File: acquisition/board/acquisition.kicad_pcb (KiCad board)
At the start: 4 copper layers, 432 parts, among them J1 XILINX_JTAG, J10 MMCX, J11 MMCX, J12 MMCX, J13 MMCX, J14 MMCX, J15 MMCX, J16 MMCX, J17 MMCX, J18 UX60SX-MB-5ST, J19 CONN_01X05, J2 MMCX, J20 CONN_01X06, J3 MMCX, J4 MMCX, J5 MMCX, J6 MMCX, J7 MMCX, J8 MMCX, J9 MMCX, Q1 SSM6N58NU, Q2 SSM6N58NU, U1 AD9251, U10 FT232HL, U11 LMK04806, U12 AK5DAF1-100.0000T2, U14 74AVCH1T45, U15 74AVCH1T45, U16 74AVCH1T45, U17 74AVCH1T45, U18 74AVCH1T45, U19 74AVCH1T45, U2 XC7A50T-1FTG256C, U20 74AVCH1T45, U21 ECS-3225MVQ-120-CN-TR, U22 93LC56B-MS, U23 74AVCH1T45, U24 74AVCH1T45, U25 LTC3374-QFN, U26 LT3042, U27 LT3042, U28 ADR510, U29 SIP32408, U3 AD9251, U30 LDO1117-12, U4 AD9251, U5 AD9251, U6 ICE40UP5K_QFN48, U7 STM32L031-QFN32, U8 S27KS0642, U9 S25FL128SAGBHIA10

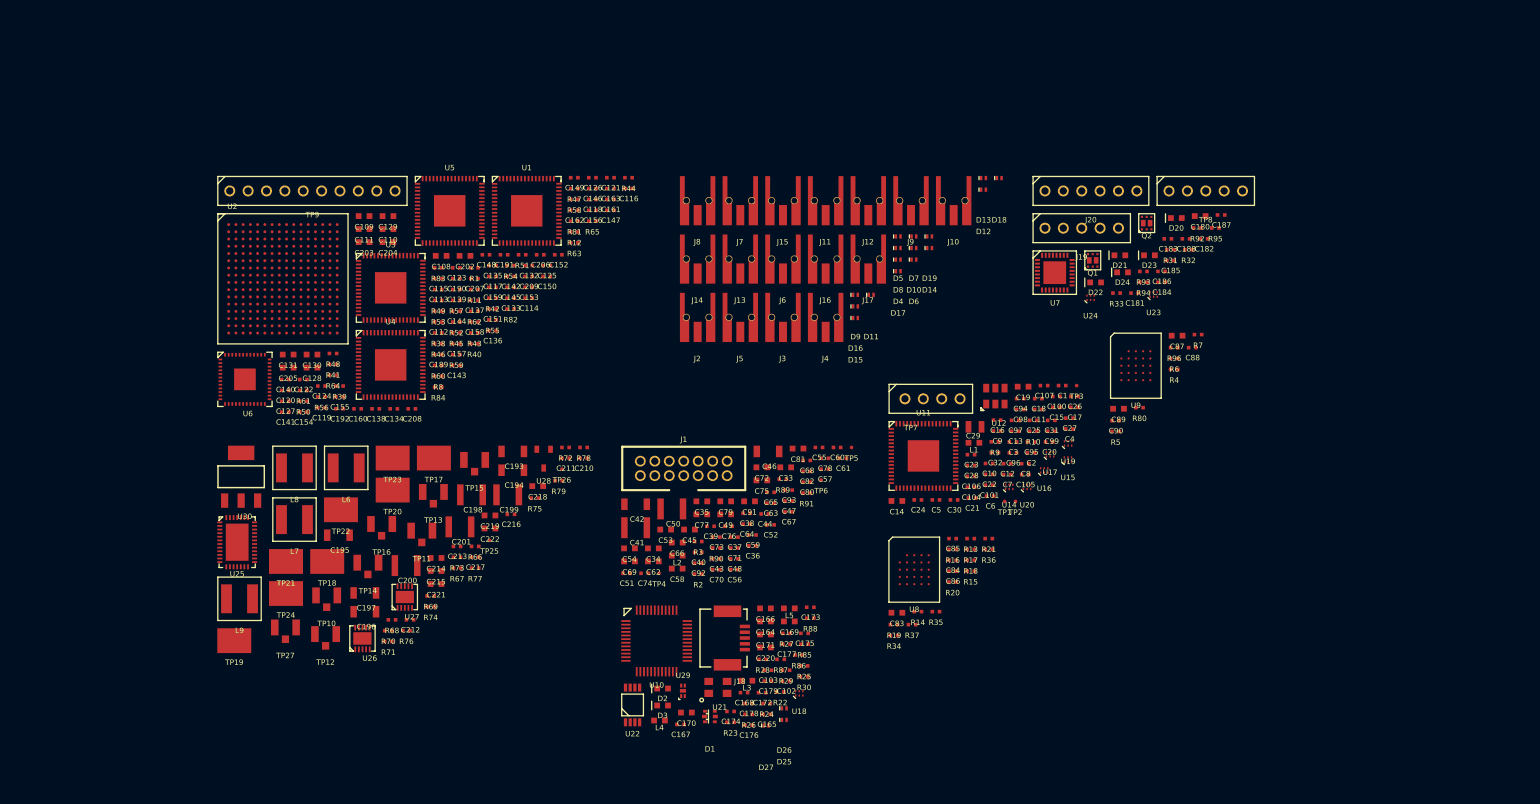
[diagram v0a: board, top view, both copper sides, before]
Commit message: Initial layout floorplanning
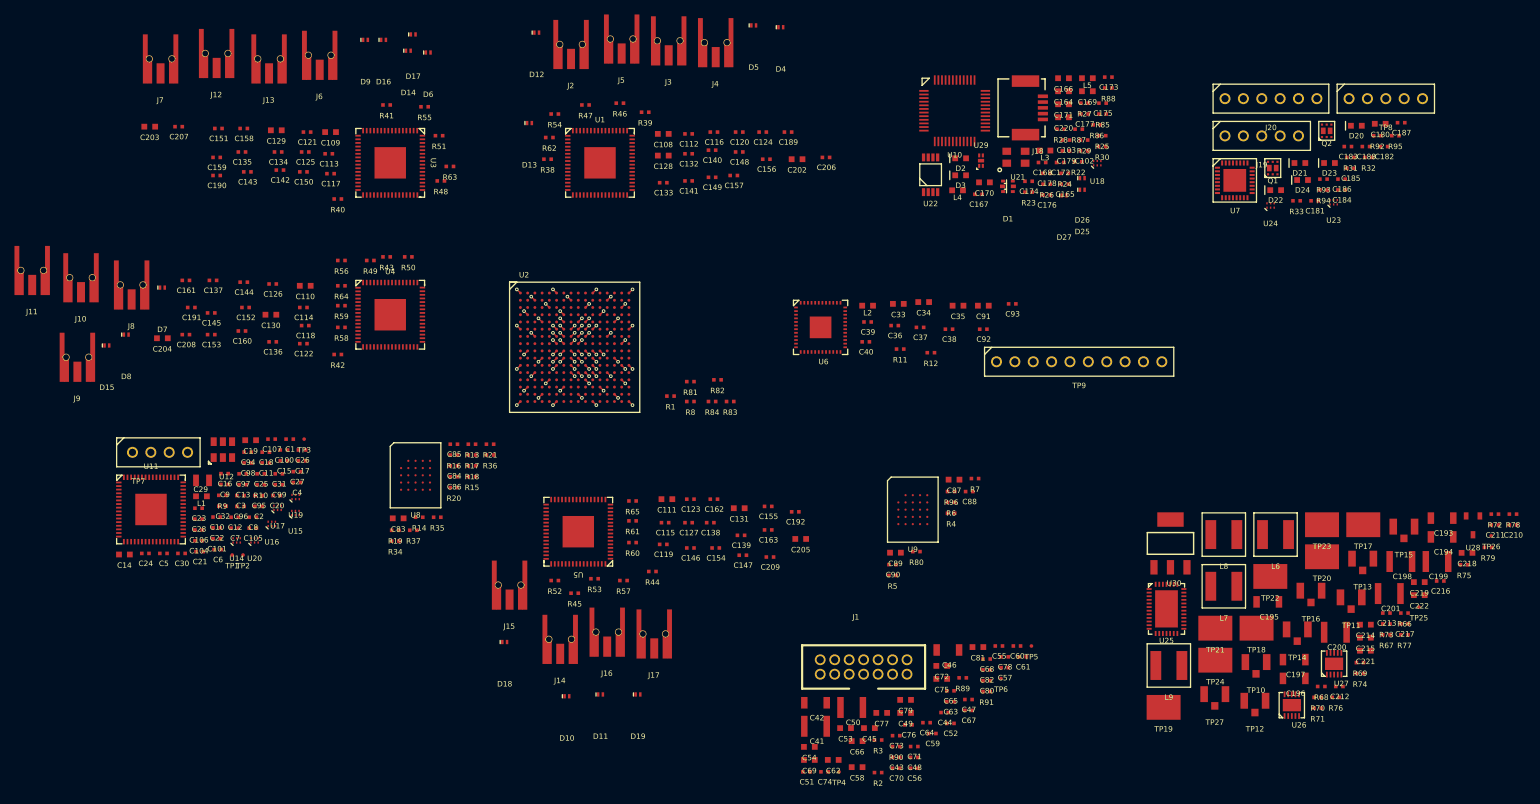
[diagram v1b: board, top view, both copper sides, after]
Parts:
- moved C193 128.8 mm to (204.4, 91.1)
- moved C194 128.8 mm to (204.4, 93.7)
- moved C198 128.8 mm to (198.7, 97.1)
- moved C199 128.8 mm to (203.7, 97.1)
- moved C200 128.8 mm to (189.7, 106.9)
- moved C201 128.8 mm to (197.1, 101.5)
- moved C210 128.8 mm to (214.2, 92.1)
- moved C211 128.8 mm to (211.7, 92.1)
- moved C213 128.8 mm to (196.7, 104.2)
- moved C216 128.8 mm to (204.2, 99.8)
- moved C217 128.8 mm to (199.2, 105.8)
- moved C218 128.8 mm to (207.9, 95.9)
- moved C219 128.8 mm to (201.3, 100.0)
- moved C222 128.8 mm to (201.3, 101.8)
- moved L6 128.8 mm to (181.4, 93.4)
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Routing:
- net /GND: track 0.00 -> 161.8 mm, vias 0 -> 40
- net /D1V8: track 0.00 -> 117.8 mm, vias 0 -> 30
- net /1V0: track 0.00 -> 43.3 mm, vias 0 -> 9
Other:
- copper layers 4 -> 6
